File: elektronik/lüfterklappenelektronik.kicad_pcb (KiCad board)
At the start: 4 copper layers, 80 x 87.6 mm, 115 parts, among them J101 Conn_01x05_Male, J102 Ckmtw_2510S-2P, J103 Conn_LAN_ENC28J60, J104 USB_B_Micro, J106 WJ2EDGRC-5.08-2P, J107 WJ2EDGRC-5.08-2P, J108 WJ2EDGRC-5.08-2P, P101 PWR_BUS_CONN1, P103 PressureSensor3, P104 PressureSensor1, P105 PressureSensor2, P109 PWR_BUS_CONN2, Q101 IRLR8743TRPBF, Q102 IRLR8743TRPBF, Q103 IRLR8743TRPBF, Q104 Q_NPN_Darlington_BEC, Q105 Q_NPN_Darlington_BEC, SW101 SW_Push, SW102 SW_Push, U101 Gabellichtschranke, U102 Gabellichtschranke, U103 Gabellichtschranke, U105 ESP32-WROOM-32E, U106 AMS1117-3.3, U107 CP2102N-A01-GQFN28

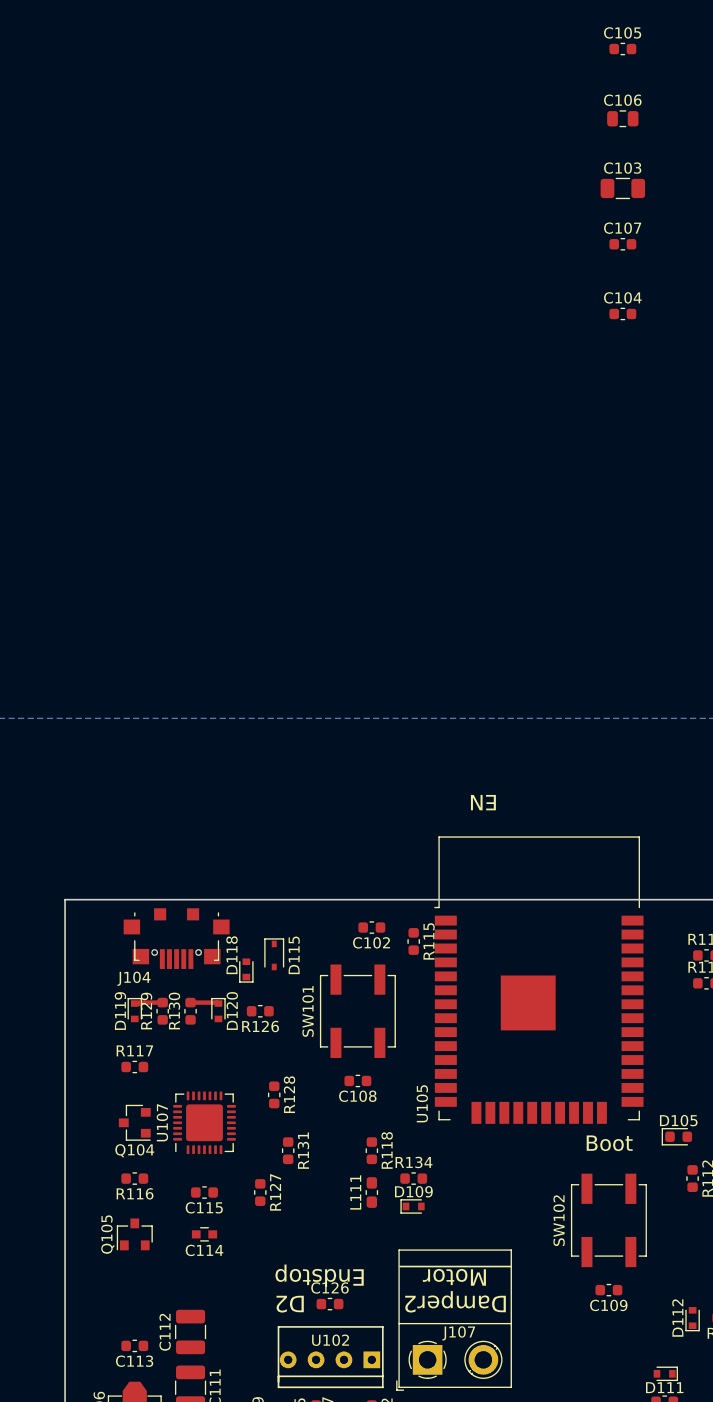
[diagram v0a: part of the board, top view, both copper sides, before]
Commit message: placing improved
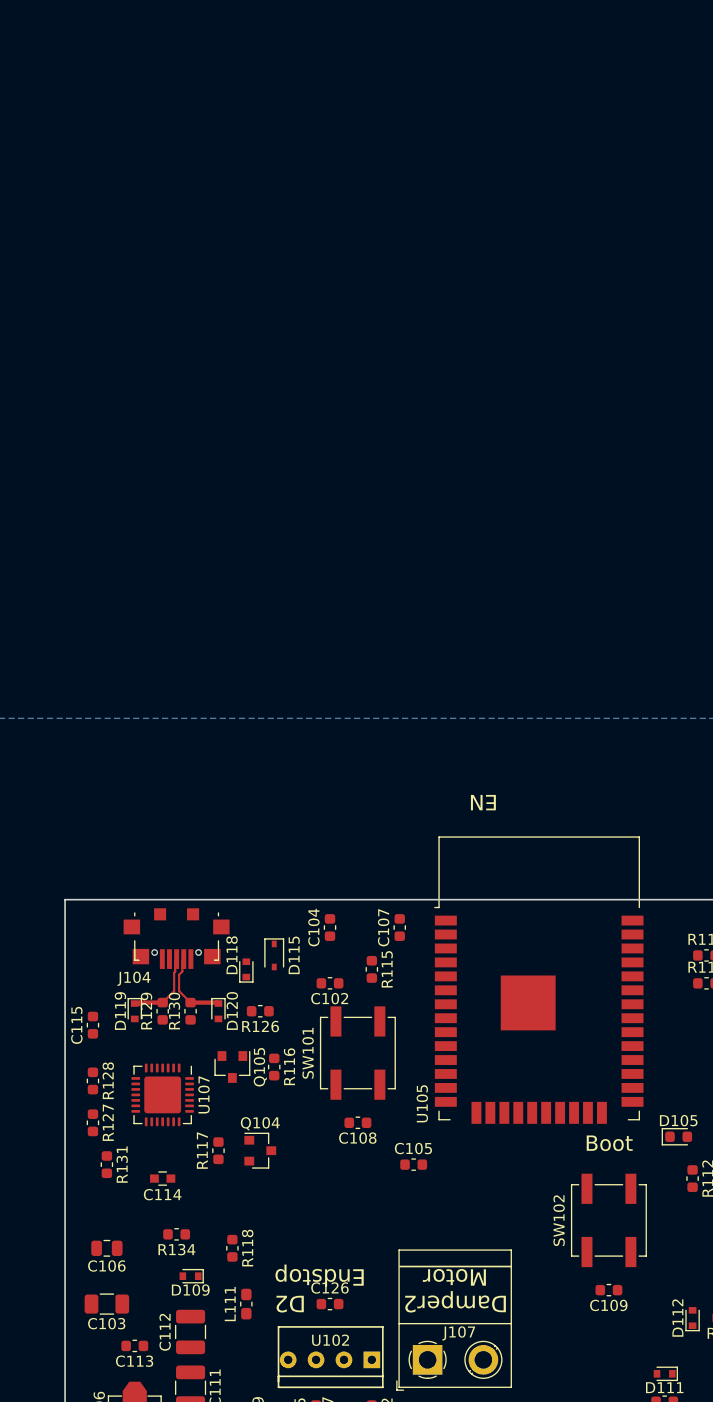
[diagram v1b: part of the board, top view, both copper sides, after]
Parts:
- moved C106 113.1 mm to (66.0, 81.3), turned to 180 degrees
- moved C103 111.9 mm to (66.0, 86.4), turned to 180 degrees
- moved C105 103.4 mm to (94.0, 73.7)
- moved C107 65.5 mm to (92.7, 52.1), turned to 90 degrees
- moved C104 61.9 mm to (86.4, 52.1), turned to 90 degrees
- moved R134 22.2 mm to (72.4, 80.0), turned to 180 degrees
- moved D109 21.3 mm to (73.7, 83.8), turned to 180 degrees
- moved C115 18.3 mm to (64.8, 61.0), turned to 90 degrees
- moved Q105 17.6 mm to (77.5, 64.8), turned to 270 degrees
- moved R128 16.6 mm to (64.8, 66.0)
- moved R131 16.6 mm to (66.0, 73.7)
- moved R127 16.5 mm to (64.8, 69.8)
- moved R116 16.3 mm to (81.3, 64.8), turned to 270 degrees
- moved R118 15.5 mm to (77.5, 81.3)
- moved L111 15.3 mm to (78.7, 86.4)
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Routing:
- net /UCD+: track 2.58 -> 7.15 mm
- net /UCD-: track 2.58 -> 7.06 mm
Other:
- net class 12V added: clearance 0.2, trace_width 0.8, via_dia 0.6, via_drill 0.4
- net class 3V3 added: clearance 0.2, trace_width 0.4, via_dia 0.6, via_drill 0.4
- net class 5V added: clearance 0.2, trace_width 0.5, via_dia 0.6, via_drill 0.4
- net class Default: trace_width 0.4 -> 0.3
